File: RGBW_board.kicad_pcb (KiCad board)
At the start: 2 copper layers, 39 x 28 mm, 13 parts, among them J1 Jack-DC, J2 Conn_01x02, J3 Conn_01x04, J4 Conn_01x02, Q1 2N7002, Q2 2N7002, Q3 2N7002, Q4 2N7002, U1 WeMos_mini

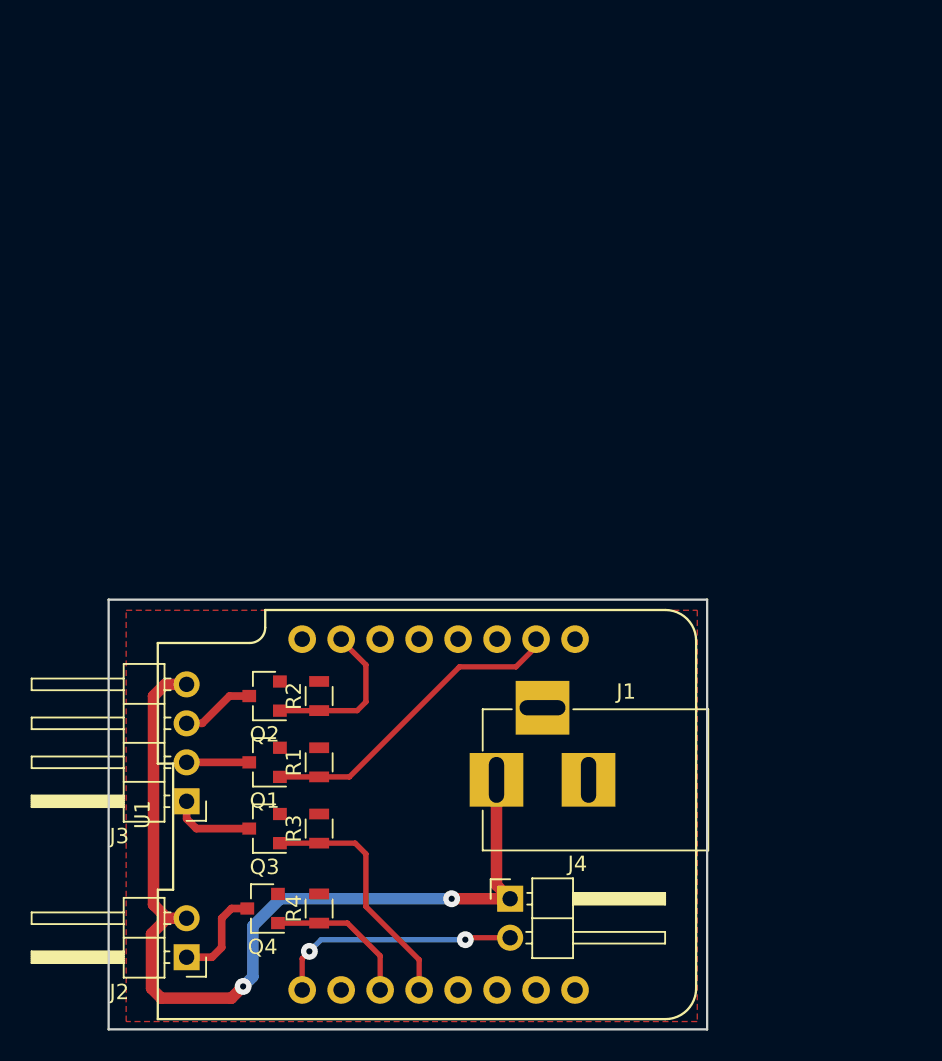
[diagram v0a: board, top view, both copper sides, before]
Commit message: --REV1-- Added rev1 to project git
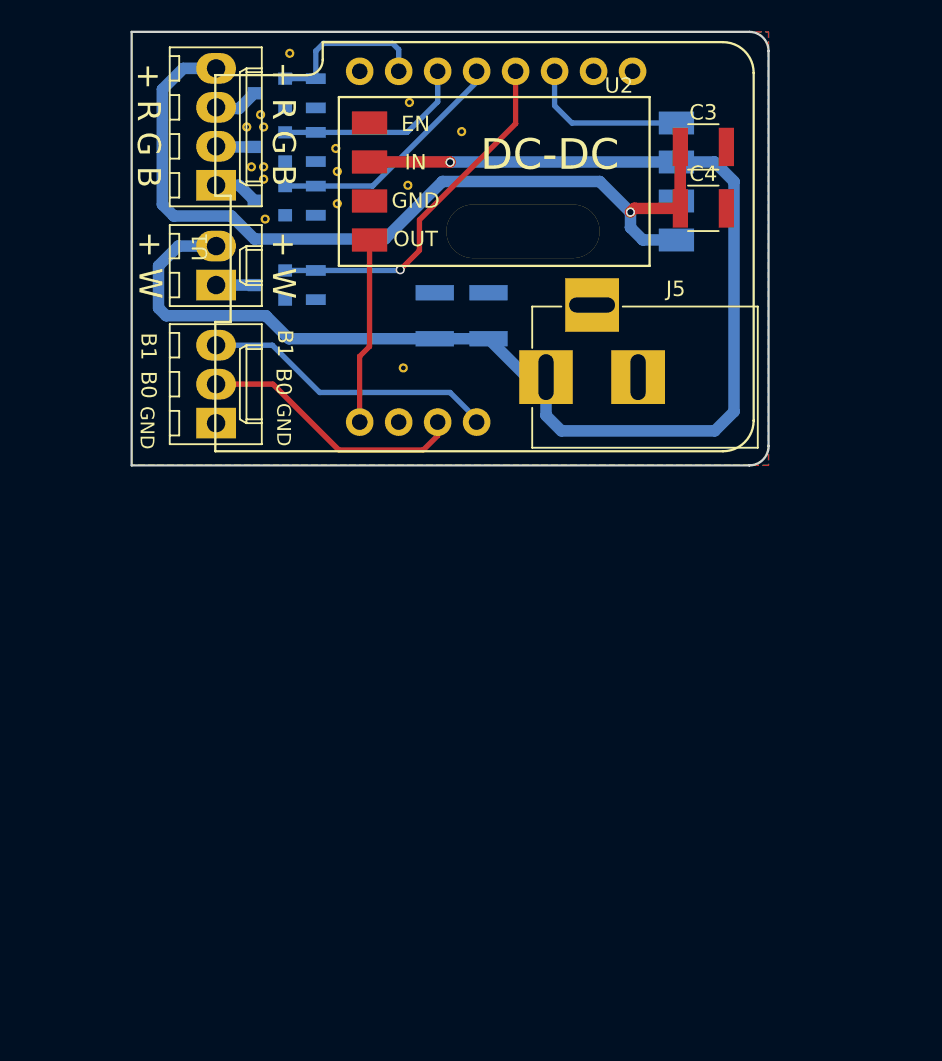
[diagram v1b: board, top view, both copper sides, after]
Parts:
- removed J2: Conn_01x02, Pin_Headers:Pin_Header_Angled_1x02_Pitch2.54mm
- added C1: C_Small, Capacitors_SMD:C_1210, B.Cu at (151.8, 72.5)
- added C2: C_Small, Capacitors_SMD:C_1210, B.Cu at (148.2, 72.5)
- added C3: C_Small, Capacitors_SMD:C_1210, F.Cu at (165.8, 61.5)
- added C4: C_Small, Capacitors_SMD:C_1210, F.Cu at (165.8, 65.5)
- added J5: Jack-DC, Connectors:BARREL_JACK, F.Cu at (155.5, 76.5)
- added REF**: via_0.6mm, kenneth:via_0.6mm, F.Cu at (136.3, 62.8)
- added REF**: via_0.6mm, kenneth:via_0.6mm, F.Cu at (141.9, 63.1)
- added REF**: via_0.6mm, kenneth:via_0.6mm, F.Cu at (137.2, 66.2)
- added REF**: via_0.6mm, kenneth:via_0.6mm, F.Cu at (141.9, 65.2)
- added REF**: via_0.6mm, kenneth:via_0.6mm, F.Cu at (146.5, 64.0)
- added REF**: via_0.6mm, kenneth:via_0.6mm, F.Cu at (150.0, 60.5)
- added REF**: via_0.6mm, kenneth:via_0.6mm, F.Cu at (146.2, 75.9)
- added REF**: via_0.6mm, kenneth:via_0.6mm, F.Cu at (137.1, 62.8)
- added REF**: via_0.6mm, kenneth:via_0.6mm, F.Cu at (137.1, 63.6)
- added REF**: via_0.6mm, kenneth:via_0.6mm, F.Cu at (136.0, 60.2)
- added REF**: via_0.6mm, kenneth:via_0.6mm, F.Cu at (137.1, 60.2)
- added REF**: via_0.6mm, kenneth:via_0.6mm, F.Cu at (136.9, 59.4)
- added REF**: via_0.6mm, kenneth:via_0.6mm, F.Cu at (138.8, 55.4)
- added REF**: via_0.6mm, kenneth:via_0.6mm, F.Cu at (146.6, 58.6)
- added REF**: via_0.6mm, kenneth:via_0.6mm, F.Cu at (141.8, 61.6)
- added U2: Mini_DC-DC_4.5-24V_to_0.8-17V, kenneth:Mini_DC-DC_converter, F.Cu at (144.0, 63.8)
- added U3: Mini_DC-DC_4.5-24V_to_0.8-17V, kenneth:Mini_DC-DC_converter, B.Cu at (164.0, 63.8)
- J1: value Jack-DC -> BTNs; footprint Connectors:BARREL_JACK -> Connectors_Molex:Molex_KK-6410-03_03x2.54mm_Straight
- J3: value Conn_01x04 -> RGB; footprint Pin_Headers:Pin_Header_Angled_1x04_Pitch2.54mm -> Connectors_Molex:Molex_KK-6410-04_04x2.54mm_Straight
- J4: value Conn_01x02 -> White; footprint Pin_Headers:Pin_Header_Angled_1x02_Pitch2.54mm -> Connectors_Molex:Molex_KK-6410-02_02x2.54mm_Straight
- Q1, Q2, Q3, Q4, R1, R2, R3, R4: moved to B.Cu
- moved J4 44.3 mm to (134.0, 70.5), turned to 90 degrees
- moved Q1 43.6 mm to (137.5, 58.0)
- moved R1 43.6 mm to (140.5, 58.0), turned to 270 degrees
- moved Q3 40.9 mm to (137.5, 65.0)
- moved R3 40.9 mm to (140.5, 65.0), turned to 270 degrees
- moved Q4 40.6 mm to (137.5, 70.5)
- moved R4 40.6 mm to (140.5, 70.5), turned to 270 degrees
- moved J3 40.2 mm to (134.0, 64.0), turned to 90 degrees
- moved U1 37.2 mm to (152.2, 68.0)
- moved Q2 35.8 mm to (137.5, 61.5)
- moved R2 35.8 mm to (140.5, 61.5), turned to 270 degrees
- moved J1 29.6 mm to (134.0, 79.5), turned to 90 degrees
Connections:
- J1 pad 1: +12V -> GND
- J1 pad 2: GND -> /BTN0
- J1 pad 3: GND -> /BTN1
- J3 pad 2: /RED_PWM_OUT -> /GREEN_PWM_OUT
- J3 pad 3: /GREEN_PWM_OUT -> /RED_PWM_OUT
- J4 pad 1: +12V -> /WHITE_PWM_OUT
- J4 pad 2: Net-(J4-Pad2) -> +24V
- U1 pad 1: Net-(J4-Pad2) -> /5V
- U1 pad 10: /RED_PWM_IN -> Net-(U1-Pad10)
- U1 pad 11: Net-(U1-Pad11) -> /Enable
- U1 pad 12: Net-(U1-Pad12) -> /WHITE_PWM_IN
- U1 pad 13: Net-(U1-Pad13) -> /BLUE_PWM_IN
- U1 pad 14: Net-(U1-Pad14) -> /GREEN_PWM_IN
- U1 pad 15: /GREEN_PWM_IN -> /RED_PWM_IN
- U1 pad 3: /WHITE_PWM_IN -> /BTN0
- U1 pad 4: /BLUE_PWM_IN -> /BTN1
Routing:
- net +24V: track 0.00 -> 89.1 mm, vias 0 -> 1
- net /BTN1: track 0.00 -> 19.2 mm
- net /BTN0: track 0.00 -> 17.5 mm
- net Net-(J4-Pad2): track 16.2 -> 0.00 mm, vias 2 -> 0
- net /WHITE_PWM_IN: track 9.77 -> 23.7 mm, vias 0 -> 1
- net /5V: track 0.00 -> 12.1 mm
- net /Enable: track 0.00 -> 10.6 mm
- net /RED_PWM_IN: track 20.7 -> 11.0 mm
- net /WHITE_PWM_OUT: track 6.38 -> 2.50 mm
- net +12V: track 59.9 -> 57.1 mm, vias 2 -> 1
- net /BLUE_PWM_OUT: track 5.49 -> 2.91 mm
- net /GREEN_PWM_OUT: track 4.82 -> 2.52 mm
- net /GREEN_PWM_IN: track 10.6 -> 12.8 mm
- net /RED_PWM_OUT: track 4.08 -> 2.95 mm
- added copper zone on B.Cu, net GND
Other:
- board size 39 x 28 mm -> 41.5 x 28.2 mm
- net class Default: clearance 0.3 -> 0.2; via_dia 1.1 -> 0.6
- net class Power: via_dia 1.1 -> 0.6
- net class Power2 removed
- rule trace_clearance: 0.3 -> 0.2
- board text added: "+ R G B"
- board text added: "+ W"
- board text added: "B0"
- board text added: "B1"
- board text added: "GND"

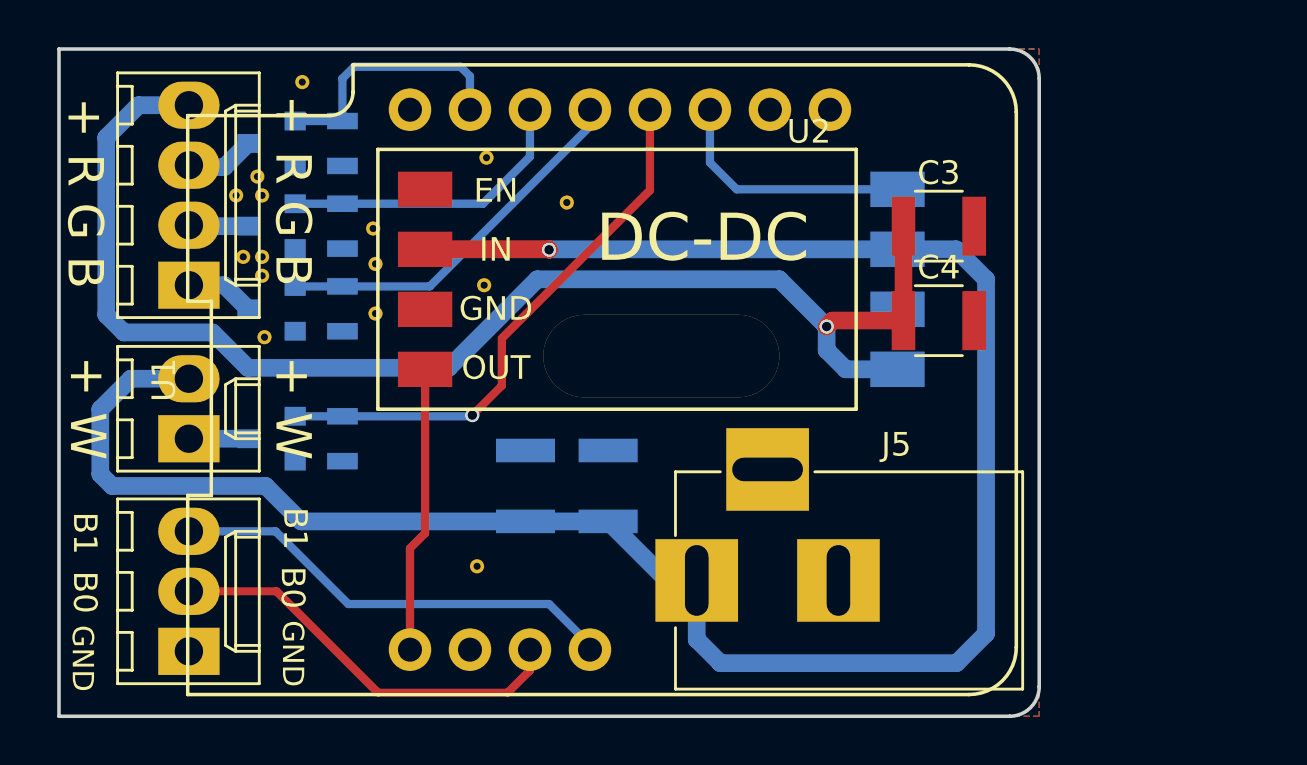
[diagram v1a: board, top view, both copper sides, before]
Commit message: --REV2-- Added rev2 to git project
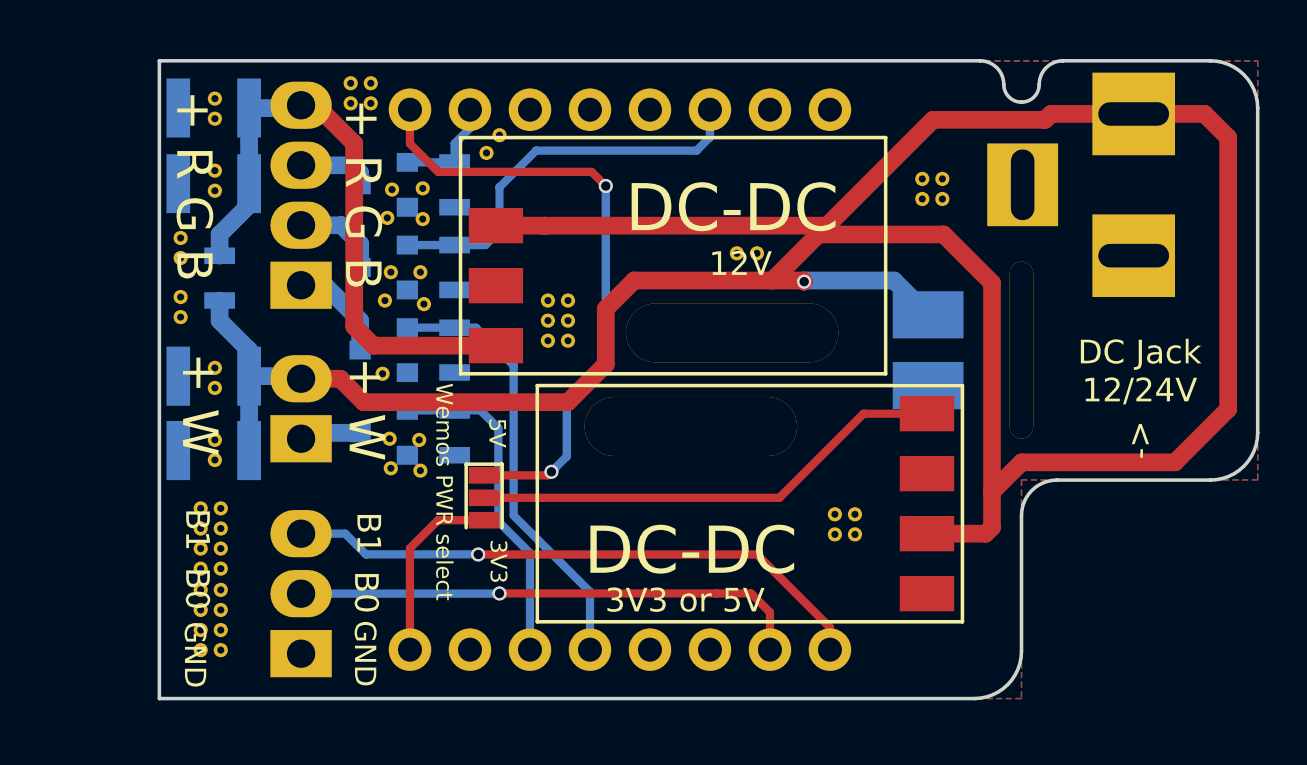
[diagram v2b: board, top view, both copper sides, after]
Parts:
- removed the REF** at (136.3, 62.8)
- removed the REF** at (141.9, 63.1)
- removed the REF** at (137.2, 66.2)
- removed the REF** at (141.9, 65.2)
- removed the REF** at (146.5, 64.0)
- removed the REF** at (146.2, 75.9)
- removed the REF** at (137.1, 62.8)
- removed the REF** at (137.1, 63.6)
- removed the REF** at (136.0, 60.2)
- removed the REF** at (137.1, 60.2)
- removed the REF** at (136.9, 59.4)
- removed the REF** at (138.8, 55.4)
- removed the REF** at (146.6, 58.6)
- removed the REF** at (141.8, 61.6)
- added J2: Conn_01x02, kenneth:Battery_wirePad_SMD, B.Cu at (165.3, 65.2)
- added JP1: Jumper_NC_Dual, kenneth:Jumper_dual, F.Cu at (146.5, 73.0)
- added JP2: Jumper_NO_Small, Resistors_SMD:R_0805, B.Cu at (135.3, 63.7)
- added REF**: via_0.6mm, kenneth:via_0.6mm, F.Cu at (135.1, 67.5)
- added REF**: via_0.6mm, kenneth:via_0.6mm, F.Cu at (165.1, 60.4)
- added REF**: via_0.6mm, kenneth:via_0.6mm, F.Cu at (165.9, 60.4)
- added REF**: via_0.6mm, kenneth:via_0.6mm, F.Cu at (165.1, 59.5)
- added REF**: via_0.6mm, kenneth:via_0.6mm, F.Cu at (143.9, 59.9)
- added REF**: via_0.6mm, kenneth:via_0.6mm, F.Cu at (142.4, 61.1)
- added REF**: via_0.6mm, kenneth:via_0.6mm, F.Cu at (143.9, 61.2)
- added REF**: via_0.6mm, kenneth:via_0.6mm, F.Cu at (142.6, 60.0)
- added REF**: via_0.6mm, kenneth:via_0.6mm, F.Cu at (142.6, 63.5)
- added REF**: via_0.6mm, kenneth:via_0.6mm, F.Cu at (143.9, 64.8)
- added REF**: via_0.6mm, kenneth:via_0.6mm, F.Cu at (142.3, 64.7)
- added REF**: via_0.6mm, kenneth:via_0.6mm, F.Cu at (135.1, 71.4)
- added REF**: via_0.6mm, kenneth:via_0.6mm, F.Cu at (143.8, 63.5)
- added REF**: via_0.6mm, kenneth:via_0.6mm, F.Cu at (142.2, 67.8)
- added REF**: via_0.6mm, kenneth:via_0.6mm, F.Cu at (143.8, 70.5)
- added REF**: via_0.6mm, kenneth:via_0.6mm, F.Cu at (142.6, 71.8)
- added REF**: via_0.6mm, kenneth:via_0.6mm, F.Cu at (143.8, 71.8)
- added REF**: via_0.6mm, kenneth:via_0.6mm, F.Cu at (142.5, 70.5)
- added REF**: via_0.6mm, kenneth:via_0.6mm, F.Cu at (161.3, 73.7)
- added REF**: via_0.6mm, kenneth:via_0.6mm, F.Cu at (162.2, 74.5)
- added REF**: via_0.6mm, kenneth:via_0.6mm, F.Cu at (161.3, 74.5)
- added REF**: via_0.6mm, kenneth:via_0.6mm, F.Cu at (162.2, 73.7)
- added REF**: via_0.6mm, kenneth:via_0.6mm, F.Cu at (135.1, 68.3)
- added REF**: via_0.6mm, kenneth:via_0.6mm, F.Cu at (141.7, 55.5)
- added REF**: via_0.6mm, kenneth:via_0.6mm, F.Cu at (140.8, 56.3)
- added REF**: via_0.6mm, kenneth:via_0.6mm, F.Cu at (141.7, 56.3)
- added REF**: via_0.6mm, kenneth:via_0.6mm, F.Cu at (140.8, 55.5)
- added REF**: via_0.6mm, kenneth:via_0.6mm, F.Cu at (146.6, 58.4)
- added REF**: via_0.6mm, kenneth:via_0.6mm, F.Cu at (147.2, 57.6)
- added REF**: via_0.6mm, kenneth:via_0.6mm, F.Cu at (135.3, 76.9)
- added REF**: via_0.6mm, kenneth:via_0.6mm, F.Cu at (134.5, 77.8)
- added REF**: via_0.6mm, kenneth:via_0.6mm, F.Cu at (135.3, 77.8)
- added REF**: via_0.6mm, kenneth:via_0.6mm, F.Cu at (134.5, 76.9)
- added REF**: via_0.6mm, kenneth:via_0.6mm, F.Cu at (135.1, 70.5)
- added REF**: via_0.6mm, kenneth:via_0.6mm, F.Cu at (134.5, 78.6)
- added REF**: via_0.6mm, kenneth:via_0.6mm, F.Cu at (135.3, 79.5)
- added REF**: via_0.6mm, kenneth:via_0.6mm, F.Cu at (134.5, 79.5)
- added REF**: via_0.6mm, kenneth:via_0.6mm, F.Cu at (135.3, 78.6)
- added REF**: via_0.6mm, kenneth:via_0.6mm, F.Cu at (135.3, 75.2)
- added REF**: via_0.6mm, kenneth:via_0.6mm, F.Cu at (134.5, 76.0)
- added REF**: via_0.6mm, kenneth:via_0.6mm, F.Cu at (135.3, 76.0)
- added REF**: via_0.6mm, kenneth:via_0.6mm, F.Cu at (134.5, 75.2)
- added REF**: via_0.6mm, kenneth:via_0.6mm, F.Cu at (134.5, 73.5)
- added REF**: via_0.6mm, kenneth:via_0.6mm, F.Cu at (135.3, 74.3)
- added REF**: via_0.6mm, kenneth:via_0.6mm, F.Cu at (135.1, 59.1)
- added REF**: via_0.6mm, kenneth:via_0.6mm, F.Cu at (134.5, 74.3)
- added REF**: via_0.6mm, kenneth:via_0.6mm, F.Cu at (135.3, 73.5)
- added REF**: via_0.6mm, kenneth:via_0.6mm, F.Cu at (133.7, 62.0)
- added REF**: via_0.6mm, kenneth:via_0.6mm, F.Cu at (133.7, 65.3)
- added REF**: via_0.6mm, kenneth:via_0.6mm, F.Cu at (133.7, 62.9)
- added REF**: via_0.6mm, kenneth:via_0.6mm, F.Cu at (133.7, 64.5)
- added REF**: via_0.6mm, kenneth:via_0.6mm, F.Cu at (157.2, 62.6)
- added REF**: via_0.6mm, kenneth:via_0.6mm, F.Cu at (158.1, 62.6)
- added REF**: via_0.6mm, kenneth:via_0.6mm, F.Cu at (150.1, 64.7)
- added REF**: via_0.6mm, kenneth:via_0.6mm, F.Cu at (149.2, 64.7)
- added REF**: via_0.6mm, kenneth:via_0.6mm, F.Cu at (135.1, 57.0)
- added REF**: via_0.6mm, kenneth:via_0.6mm, F.Cu at (149.2, 65.5)
- added REF**: via_0.6mm, kenneth:via_0.6mm, F.Cu at (150.1, 66.3)
- added REF**: via_0.6mm, kenneth:via_0.6mm, F.Cu at (149.2, 66.3)
- added REF**: via_0.6mm, kenneth:via_0.6mm, F.Cu at (150.1, 65.5)
- added REF**: via_0.6mm, kenneth:via_0.6mm, F.Cu at (135.1, 60.0)
- added REF**: via_0.6mm, kenneth:via_0.6mm, F.Cu at (135.1, 56.1)
- added REF**: via_0.6mm, kenneth:via_0.6mm, F.Cu at (165.9, 59.5)
- C3, C4, J5: moved to B.Cu
- U2: footprint kenneth:Mini_DC-DC_converter -> kenneth:Mini_DC-DC_converter_RED
- U3: footprint kenneth:Mini_DC-DC_converter -> kenneth:Mini_DC-DC_converter_RED; moved to F.Cu
- moved C4 32.0 mm to (135.1, 56.5), turned to 180 degrees
- moved C3 30.8 mm to (135.1, 59.7), turned to 180 degrees
- moved J5 27.1 mm to (174.0, 56.8), turned to 90 degrees
- moved U2 23.3 mm to (165.2, 73.2), turned to 180 degrees
- moved REF** 20.2 mm to (169.2, 66.8)
- moved C1 17.3 mm to (135.1, 67.8), turned to 180 degrees
- moved U3 17.0 mm to (147.0, 62.8), turned to 0 degrees
- moved C2 13.3 mm to (135.1, 71.0), turned to 180 degrees
- moved Q1 5.06 mm to (142.2, 59.8)
- moved Q2 5.06 mm to (142.2, 63.2)
- moved Q3 5.06 mm to (142.2, 66.8)
- moved R1 5.06 mm to (145.2, 59.8)
- moved R2 5.06 mm to (145.2, 63.2)
- moved R3 5.06 mm to (145.2, 66.8)
- moved Q4 4.76 mm to (142.2, 70.2)
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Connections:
- REF** pad : GND -> (no net)
- U1 pad 1: /5V -> Net-(JP1-Pad3)
- U1 pad 11: /Enable -> /GREEN_PWM_IN
- U1 pad 12: /WHITE_PWM_IN -> Net-(U1-Pad12)
- U1 pad 13: /BLUE_PWM_IN -> Net-(U1-Pad13)
- U1 pad 14: /GREEN_PWM_IN -> Net-(U1-Pad14)
- U1 pad 3: /BTN0 -> /WHITE_PWM_IN
- U1 pad 4: /BTN1 -> /BLUE_PWM_IN
- U2 pad 4: /5V -> /5Vor3V3
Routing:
- net +24V: track 89.1 -> 121.3 mm
- net +12V: track 57.1 -> 26.0 mm, vias 1 -> 0
- net Net-(JP1-Pad1): track 0.00 -> 26.4 mm, vias 0 -> 2
- net /5Vor3V3: track 0.00 -> 20.2 mm
- net /5V: track 12.1 -> 0.00 mm
- net /Enable: track 10.6 -> 0.00 mm
- net /WHITE_PWM_IN: track 23.7 -> 14.1 mm, vias 1 -> 0
- net Net-(JP1-Pad3): track 0.00 -> 7.92 mm
- net /RED_PWM_IN: track 11.0 -> 4.71 mm
- net /BTN1: track 19.2 -> 25.0 mm, vias 0 -> 1
- net /BTN0: track 17.5 -> 21.8 mm, vias 0 -> 1
- net /GREEN_PWM_IN: track 12.8 -> 17.0 mm
- net /BLUE_PWM_IN: track 16.0 -> 18.5 mm
- net /BLUE_PWM_OUT: track 2.91 -> 4.37 mm
- net /GREEN_PWM_OUT: track 2.52 -> 3.83 mm
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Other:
- board size 41.5 x 28.2 mm -> 46.5 x 27 mm
- net class Default: clearance 0.2 -> 0.25
- rule trace_clearance: 0.2 -> 0.25
- board text added: "->"
- board text added: "12V"
- board text added: "3V3"
- board text added: "3V3 or 5V"
- board text added: "5V"
- board text added: "DC Jack 12/24V"
- board text added: "Designed by: KKL"
- board text added: "REV1"
- board text added: "RGBW Wemos shield"
- board text added: "Wemos PWR select"
